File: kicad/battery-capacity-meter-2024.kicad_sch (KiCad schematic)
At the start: 64 parts, among them J1 PWR, J2 GND, J3 Conn_MainBoard, J4 Conn_DisplayBoard, Q1 2N3904, Q2 2N3906, Q3 2SD2390, SW1 SW_CHARGE/DISCHARGE, SW2 1A MODE, U1 LM2596_StepDown_Module, U10 AO3406, U2 LM358, U3 TM1637Display, U5 AO3406, U6 TL431LP, U7 Arduino_pro_mini, U8 TP4056, U9 AO3406

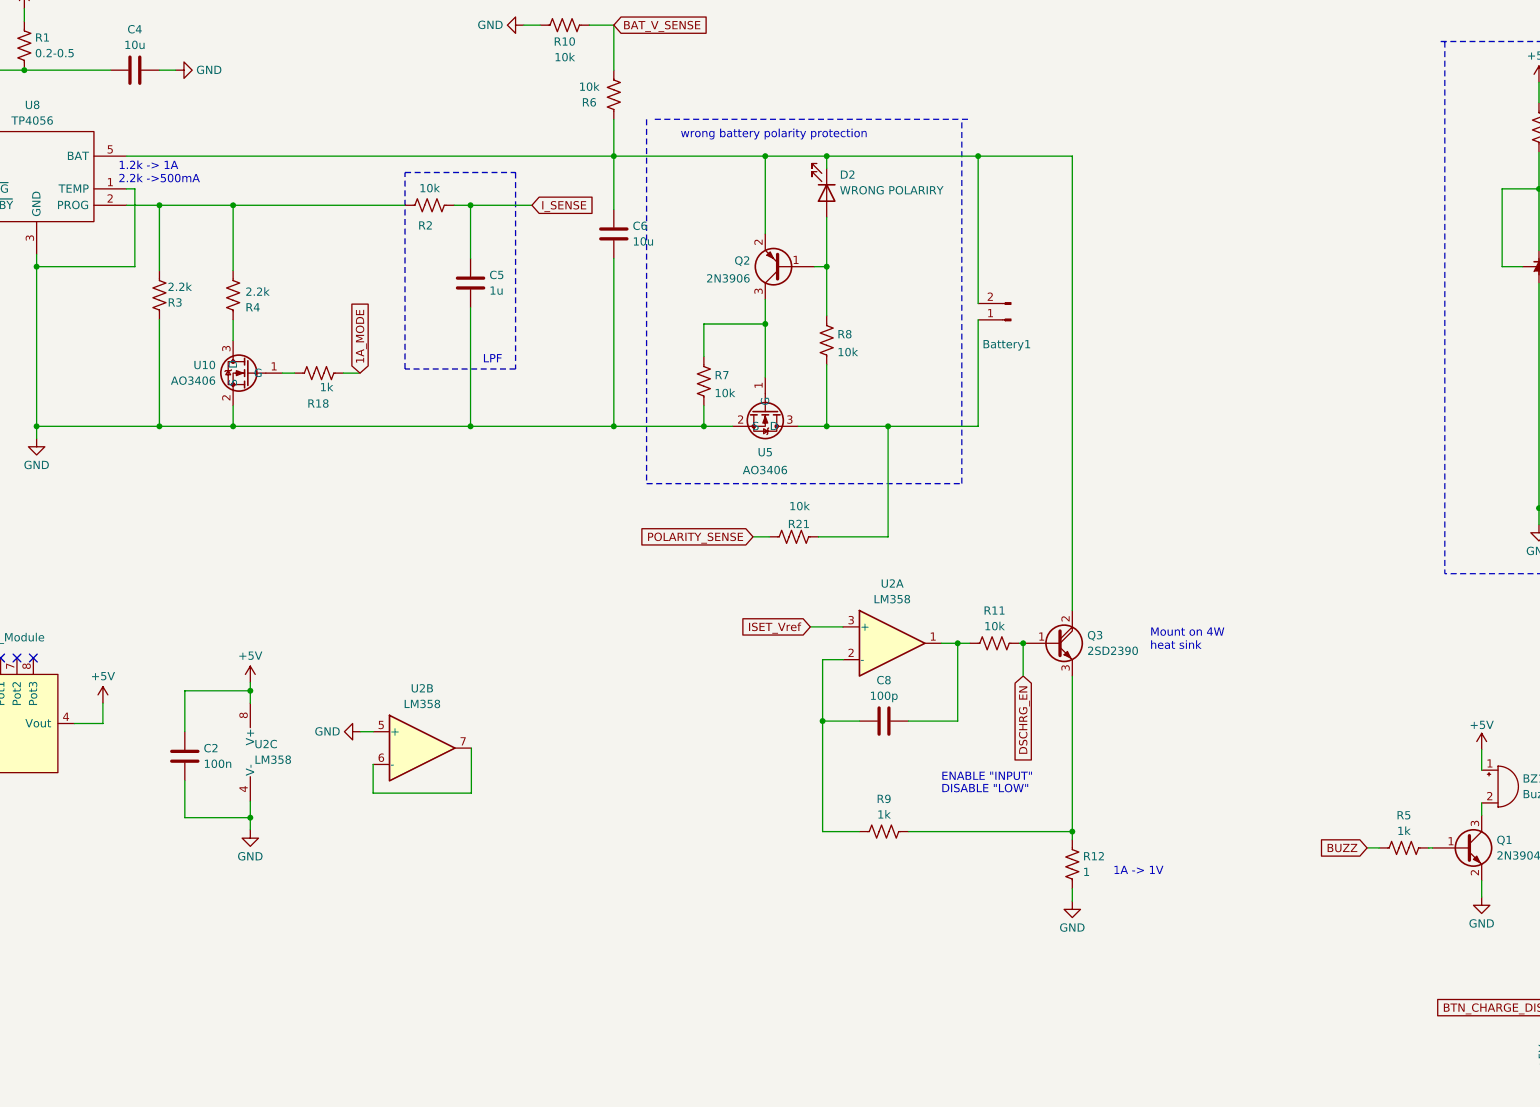
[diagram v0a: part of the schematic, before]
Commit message: add ovp
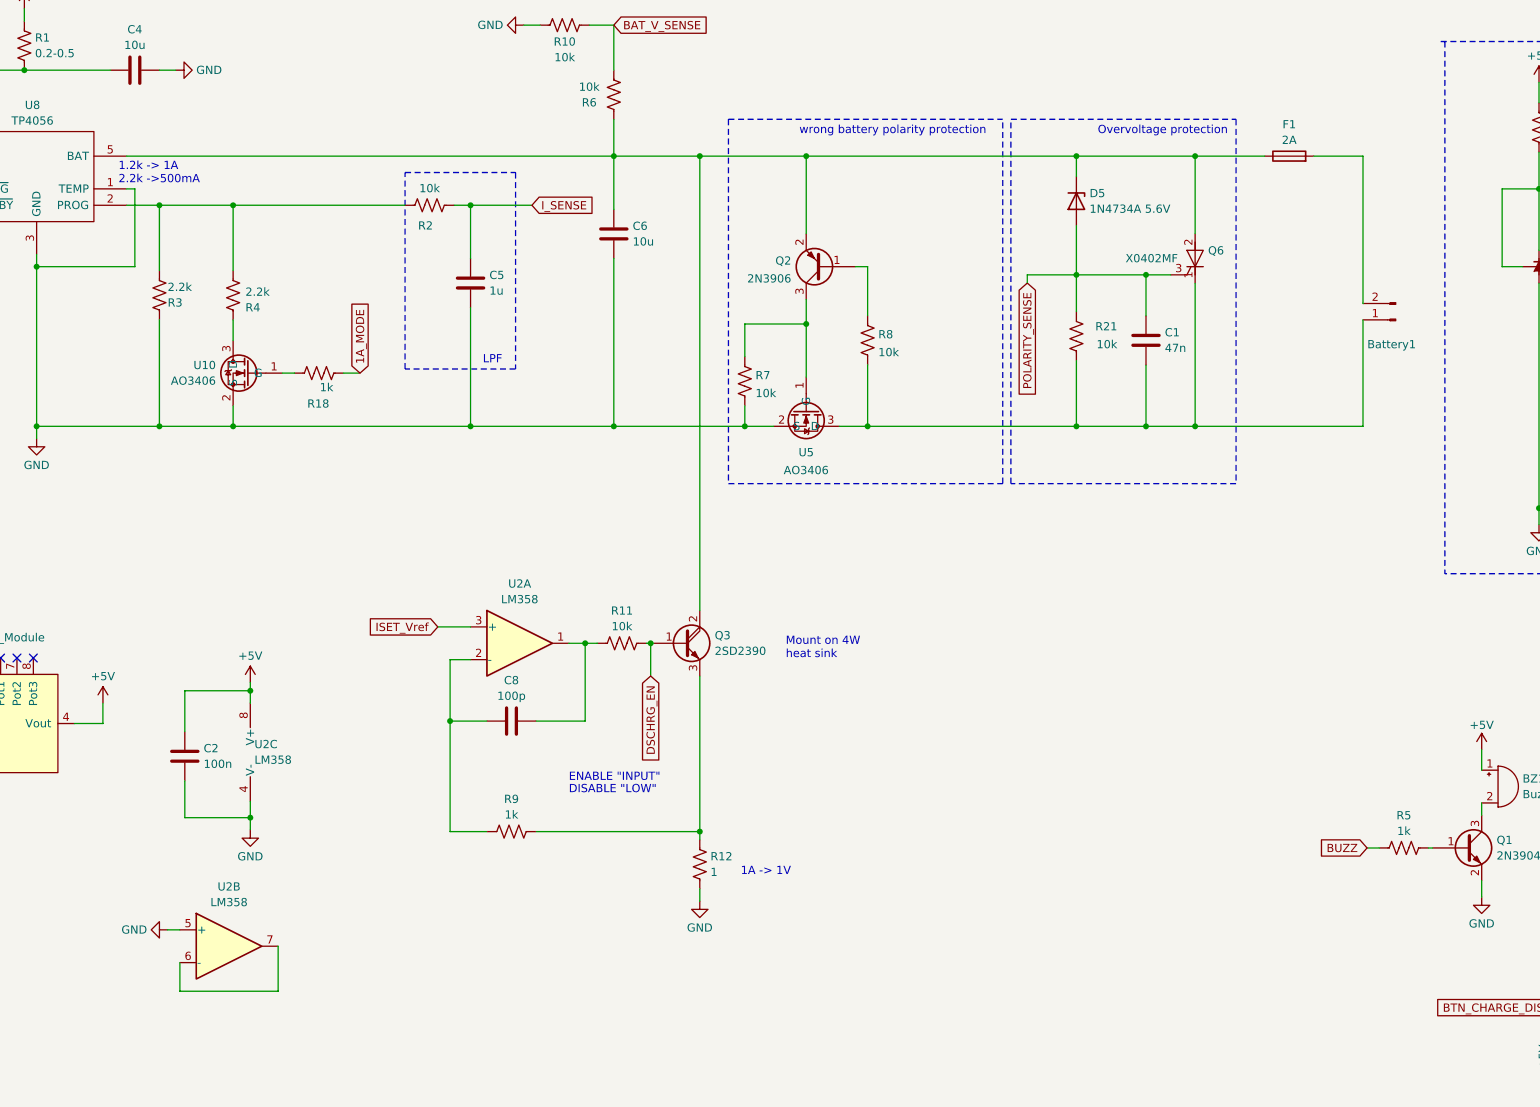
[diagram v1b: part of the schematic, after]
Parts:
- removed D2: WRONG POLARIRY, LED_THT:LED_D5.0mm, symbol Device:LED
- added C1: 47n, Capacitor_SMD:C_1206_3216Metric, symbol Device:C
- added D5: 1N4734A 5.6V, Diode_THT:D_DO-35_SOD27_P5.08mm_Vertical_KathodeUp, symbol Device:D_Zener
- added F1: 2A, Resistor_THT:R_Axial_DIN0309_L9.0mm_D3.2mm_P2.54mm_Vertical, symbol Device:Fuse
- added Q6: X0402MF, Package_TO_SOT_THT:TO-220-3_Vertical, symbol Triac_Thyristor:X0202NN
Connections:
- net POLARITY_SENSE: now also R21.1, C1.1, D5.2 (A), Q6.3 (G); no longer R21.2
- net at Battery1.1 (Pin_1), R8.1, U5.3 (D): now also R21.2, C1.2, Q6.1 (K); no longer R21.1
- net at C6.1, Q2.2 (E), Q3.2 (C)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: now also D5.1 (K), F1.1, Q6.2 (A), Q6.4 (A); no longer Battery1.2 (Pin_2)
- new net: Battery1.2 (Pin_2), F1.2
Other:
- note added: "Overvoltage protection"
- moved on the sheet: Battery1, C8, Q2, Q3, R11, R12, R21, R7, R8, R9, U2A, U2B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
